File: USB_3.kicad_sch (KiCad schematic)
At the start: 0 parts

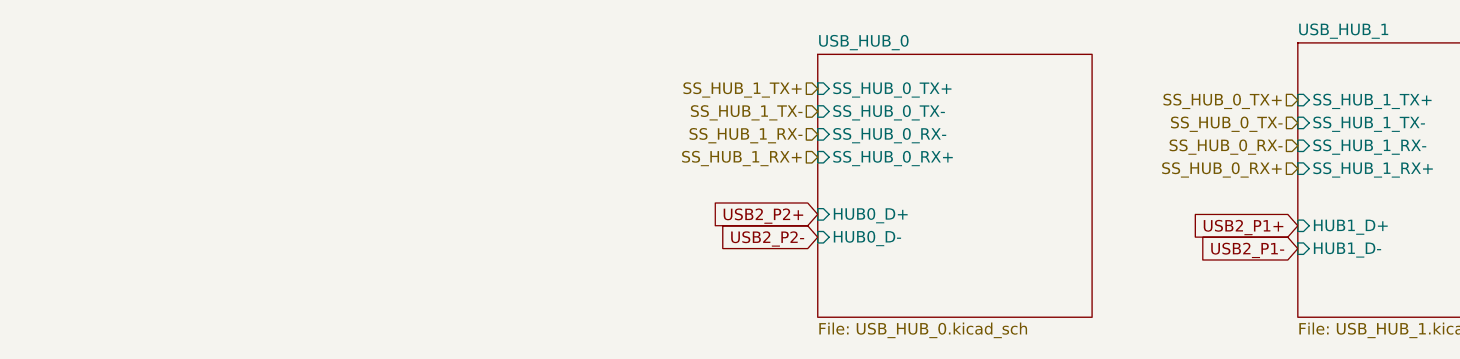
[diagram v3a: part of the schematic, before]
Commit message: .
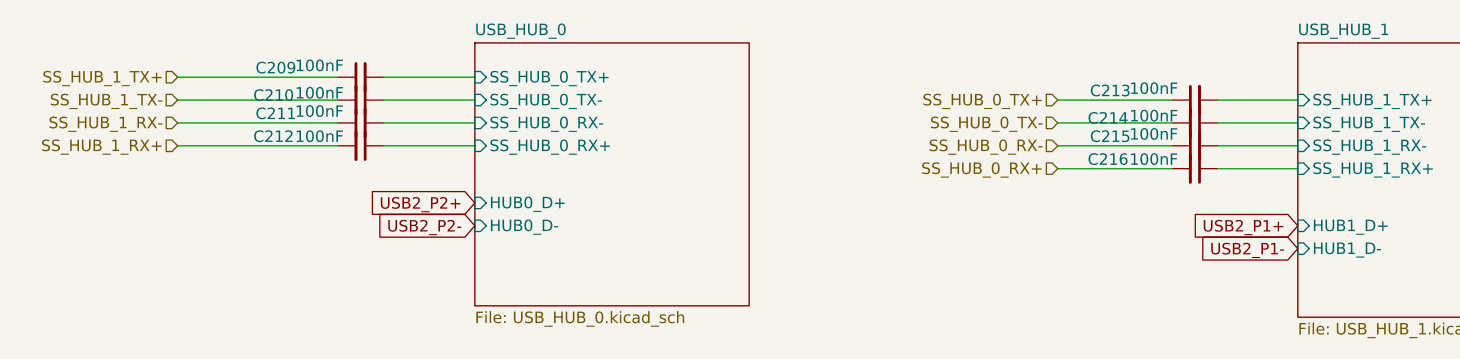
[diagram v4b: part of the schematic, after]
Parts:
- added C209, C210, C211, C212, C213, C214, C215, C216: 100nF, Capacitor_SMD:C_0402_1005Metric, symbol Device:C_Small
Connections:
- net SS_HUB_0_RX+: now also C216.2
- net SS_HUB_0_RX-: now also C215.1
- net SS_HUB_0_TX+: now also C213.1
- net SS_HUB_0_TX-: now also C214.2
- net SS_HUB_1_RX+: now also C212.2
- net SS_HUB_1_RX-: now also C211.1
- net SS_HUB_1_TX+: now also C209.1
- net SS_HUB_1_TX-: now also C210.2
- new net USB_HUB_0/SS_HUB_0_RX+: C212.1
- new net USB_HUB_0/SS_HUB_0_RX-: C211.2
- new net USB_HUB_0/SS_HUB_0_TX+: C209.2
- new net USB_HUB_0/SS_HUB_0_TX-: C210.1
- new net USB_HUB_1/SS_HUB_1_RX+: C216.1
- new net USB_HUB_1/SS_HUB_1_RX-: C215.2
- new net USB_HUB_1/SS_HUB_1_TX+: C213.2
- new net USB_HUB_1/SS_HUB_1_TX-: C214.1
